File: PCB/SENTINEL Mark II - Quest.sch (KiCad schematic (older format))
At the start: 22 parts, among them J10 External, J7 SERVO1, J8 SERVO2, J9 SENSOR, U3 STM32F103CBTx, Y1 8MHz/20pF

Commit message: Footprint Assigned
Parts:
- C11, C12, C13, C14, C15, C16, C17: footprint (none) -> Capacitor_SMD:C_0805_2012Metric
- D4: footprint (none) -> LED_SMD:LED_0805_2012Metric
- FB2, FB3, FB4: footprint (none) -> Inductor_SMD:L_0805_2012Metric
- J10: footprint (none) -> Connector_PinHeader_2.54mm:PinHeader_1x04_P2.54mm_Vertical
- J7, J8, JP1: footprint (none) -> Connector_PinHeader_2.54mm:PinHeader_1x03_P2.54mm_Vertical
- J9: footprint (none) -> Connector_PinHeader_2.54mm:PinHeader_1x09_P2.54mm_Horizontal
- R12, R7, R8, R9: footprint (none) -> Resistor_SMD:R_0805_2012Metric
- Y1: footprint (none) -> Crystal:Crystal_SMD_3225-4Pin_3.2x2.5mm_HandSoldering; symbol Device:Crystal -> Device:Crystal_GND24
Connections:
- net GND: now also C11.1, C12.1, Y1.2, Y1.4; no longer C11.2, C12.2
- net at U3.5 (PD0), Y1.1: now also C12.2; no longer C11.1
- new net: C11.2, U3.6 (PD1), Y1.3
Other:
- moved on the sheet: C11, C12
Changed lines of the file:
@@
 F 0 "C15" H 7040 2296 50  0000 L CNN
 F 1 "1uF" H 7040 2205 50  0000 L CNN
-F 2 "" H 6963 2100 50  0001 C CNN
+F 2 "Capacitor_SMD:C_0805_2012Metric" H 6963 2100 50  0001 C CNN
 F 3 "~" H 6925 2250 50  0001 C CNN
 	1    6925 2250
@@
 F 0 "C16" H 7565 2296 50  0000 L CNN
 F 1 "1uF" H 7565 2205 50  0000 L CNN
-F 2 "" H 7488 2100 50  0001 C CNN
+F 2 "Capacitor_SMD:C_0805_2012Metric" H 7488 2100 50  0001 C CNN
 F 3 "~" H 7450 2250 50  0001 C CNN
 	1    7450 2250
@@
 F 0 "C17" H 8065 2296 50  0000 L CNN
 F 1 "1uF" H 8065 2205 50  0000 L CNN
-F 2 "" H 7988 2100 50  0001 C CNN
+F 2 "Capacitor_SMD:C_0805_2012Metric" H 7988 2100 50  0001 C CNN
 F 3 "~" H 7950 2250 50  0001 C CNN
 	1    7950 2250
@@
 F 0 "C14" H 6515 2296 50  0000 L CNN
 F 1 "1uF" H 6515 2205 50  0000 L CNN
-F 2 "" H 6438 2100 50  0001 C CNN
+F 2 "Capacitor_SMD:C_0805_2012Metric" H 6438 2100 50  0001 C CNN
 F 3 "~" H 6400 2250 50  0001 C CNN
 	1    6400 2250
@@
 F 0 "R8" H 5050 1675 50  0000 L CNN
 F 1 "10K" V 5000 1575 50  0000 L CNN
-F 2 "" V 4930 1650 50  0001 C CNN
+F 2 "Resistor_SMD:R_0805_2012Metric" V 4930 1650 50  0001 C CNN
 F 3 "~" H 5000 1650 50  0001 C CNN
 	1    5000 1650
@@
 Wire Wire Line
 	5000 3700 5000 3600
-Wire Wire Line
-	4375 3700 5000 3700
-Wire Wire Line
-	4375 3400 5000 3400
-$Comp
-L Device:Crystal Y1
+$Comp
+L Device:Crystal_GND24 Y1
 U 1 1 5F6E91F4
-P 4375 3550
+P 4425 3550
 AR Path="/5F6E91F4" Ref="Y1"  Part="1"
 AR Path="/5F584CC7/5F6E91F4" Ref="Y?"  Part="1"
-F 0 "Y1" V 4329 3681 50  0000 L CNN
-F 1 "8MHz/20pF" V 4420 3681 50  0000 L CNN
-F 2 "" H 4375 3550 50  0001 C CNN
-F 3 "~" H 4375 3550 50  0001 C CNN
-	1    4375 3550
+F 0 "Y1" V 4450 2800 50  0000 L CNN
+F 1 "8MHz/20pF" V 4525 2800 50  0000 L CNN
+F 2 "Crystal:Crystal_SMD_3225-4Pin_3.2x2.5mm_HandSoldering" H 4425 3550 50  0001 C CNN
+F 3 "~" H 4425 3550 50  0001 C CNN
+	1    4425 3550
 	0    1    1    0
 $EndComp
@@
 L Device:C C11
 U 1 1 5F6E91FA
-P 4125 3400
+P 4275 3850
 AR Path="/5F6E91FA" Ref="C11"  Part="1"
 AR Path="/5F584CC7/5F6E91FA" Ref="C?"  Part="1"
-F 0 "C11" V 3925 3400 50  0000 C CNN
-F 1 "33pF" V 4000 3400 50  0000 C CNN
-F 2 "" H 4163 3250 50  0001 C CNN
-F 3 "~" H 4125 3400 50  0001 C CNN
-	1    4125 3400
-	0    1    1    0
+F 0 "C11" V 4075 3850 50  0000 C CNN
+F 1 "33pF" V 4150 3850 50  0000 C CNN
+F 2 "Capacitor_SMD:C_0805_2012Metric" H 4313 3700 50  0001 C CNN
+F 3 "~" H 4275 3850 50  0001 C CNN
+	1    4275 3850
+	0    -1   -1   0
 $EndComp
 $Comp
 L Device:C C12
 U 1 1 5F6E9200
-P 4125 3700
+P 4275 3225
 AR Path="/5F6E9200" Ref="C12"  Part="1"
 AR Path="/5F584CC7/5F6E9200" Ref="C?"  Part="1"
-F 0 "C12" V 4275 3700 50  0000 C CNN
-F 1 "33pF" V 4350 3700 50  0000 C CNN
-F 2 "" H 4163 3550 50  0001 C CNN
-F 3 "~" H 4125 3700 50  0001 C CNN
-	1    4125 3700
-	0    1    1    0
+F 0 "C12" V 4425 3225 50  0000 C CNN
+F 1 "33pF" V 4500 3225 50  0000 C CNN
+F 2 "Capacitor_SMD:C_0805_2012Metric" H 4313 3075 50  0001 C CNN
+F 3 "~" H 4275 3225 50  0001 C CNN
+	1    4275 3225
+	0    -1   -1   0
 $EndComp
 $Comp
@@
 F 0 "C13" H 5915 2071 50  0000 L CNN
 F 1 "100nF" H 5915 1980 50  0000 L CNN
-F 2 "" H 5838 1875 50  0001 C CNN
+F 2 "Capacitor_SMD:C_0805_2012Metric" H 5838 1875 50  0001 C CNN
 F 3 "~" H 5800 2025 50  0001 C CNN
 	1    5800 2025
@@
 F 0 "R9" H 5850 1775 50  0000 L CNN
 F 1 "10K" V 5800 1650 50  0000 L CNN
-F 2 "" V 5730 1725 50  0001 C CNN
+F 2 "Resistor_SMD:R_0805_2012Metric" V 5730 1725 50  0001 C CNN
 F 3 "~" H 5800 1725 50  0001 C CNN
 	1    5800 1725
@@
 L power:GND #PWR020
 U 1 1 5F6E9221
-P 3975 3550
+P 4125 3550
 AR Path="/5F6E9221" Ref="#PWR020"  Part="1"
 AR Path="/5F584CC7/5F6E9221" Ref="#PWR?"  Part="1"
-F 0 "#PWR020" H 3975 3300 50  0001 C CNN
-F 1 "GND" H 3980 3377 50  0000 C CNN
-F 2 "" H 3975 3550 50  0001 C CNN
-F 3 "" H 3975 3550 50  0001 C CNN
-	1    3975 3550
+F 0 "#PWR020" H 4125 3300 50  0001 C CNN
+F 1 "GND" V 4125 3375 50  0000 C CNN
+F 2 "" H 4125 3550 50  0001 C CNN
+F 3 "" H 4125 3550 50  0001 C CNN
+	1    4125 3550
 	0    1    1    0
 $EndComp
-Wire Wire Line
-	3975 3400 3975 3550
-Connection ~ 3975 3550
-Wire Wire Line
-	3975 3550 3975 3700
-Wire Wire Line
-	4275 3400 4375 3400
-Connection ~ 4375 3400
-Wire Wire Line
-	4275 3700 4375 3700
-Connection ~ 4375 3700
 Text Label 5000 5100 2    50   ~ 0
 DISC
@@
 F 0 "R7" H 4700 1675 50  0000 L CNN
 F 1 "330" V 4900 1575 50  0000 L CNN
-F 2 "" V 4830 1650 50  0001 C CNN
+F 2 "Resistor_SMD:R_0805_2012Metric" V 4830 1650 50  0001 C CNN
 F 3 "~" H 4900 1650 50  0001 C CNN
 	1    4900 1650
@@
 F 0 "D4" H 4893 2166 50  0000 C CNN
 F 1 "LED" H 4893 2075 50  0000 C CNN
-F 2 "" H 4900 1950 50  0001 C CNN
+F 2 "LED_SMD:LED_0805_2012Metric" H 4900 1950 50  0001 C CNN
 F 3 "~" H 4900 1950 50  0001 C CNN
 	1    4900 1950
@@
 F 0 "J9" H 7505 3792 50  0000 L CNN
 F 1 "SENSOR" H 7505 3701 50  0000 L CNN
-F 2 "" H 7425 3750 50  0001 C CNN
+F 2 "Connector_PinHeader_2.54mm:PinHeader_1x09_P2.54mm_Horizontal" H 7425 3750 50  0001 C CNN
 F 3 "~" H 7425 3750 50  0001 C CNN
 	1    7425 3750
@@
 Wire Wire Line
 	7700 2400 7950 2400
-Text Notes 1925 3675 0    50   ~ 0
+Text Notes 1250 3650 0    50   ~ 0
 Typ. Cstray = 3pF\nCa(pF) = Cb(pF) = 2*CL(pF) - 2*Cstray(pF)\nCa = Cb = 2*20 - 2*3 = 34pF
 Wire Notes Line
-	1900 3425 3650 3425
-Wire Notes Line
-	3650 3425 3650 3700
-Wire Notes Line
-	3650 3700 1900 3700
-Wire Notes Line
-	1900 3700 1900 3425
+	1225 3400 2975 3400
+Wire Notes Line
+	2975 3400 2975 3675
+Wire Notes Line
+	2975 3675 1225 3675
+Wire Notes Line
+	1225 3675 1225 3400
 Text Label 7225 3450 2    50   ~ 0
 PWM_LED
@@
 F 0 "J8" H 2593 2892 50  0000 C CNN
 F 1 "SERVO2" H 2593 2801 50  0000 C CNN
-F 2 "" H 2675 2575 50  0001 C CNN
+F 2 "Connector_PinHeader_2.54mm:PinHeader_1x03_P2.54mm_Vertical" H 2675 2575 50  0001 C CNN
 F 3 "~" H 2675 2575 50  0001 C CNN
 	1    2675 2575
@@
 F 0 "J7" H 2593 1700 50  0000 C CNN
 F 1 "SERVO1" H 2593 1791 50  0000 C CNN
-F 2 "" H 2675 2025 50  0001 C CNN
+F 2 "Connector_PinHeader_2.54mm:PinHeader_1x03_P2.54mm_Vertical" H 2675 2025 50  0001 C CNN
 F 3 "~" H 2675 2025 50  0001 C CNN
 	1    2675 2025
@@
 F 0 "FB4" V 6975 1575 50  0000 C CNN
 F 1 "1A" V 7050 1575 50  0000 C CNN
-F 2 "" V 7055 1675 50  0001 C CNN
+F 2 "Inductor_SMD:L_0805_2012Metric" V 7055 1675 50  0001 C CNN
 F 3 "~" H 7125 1675 50  0001 C CNN
 	1    7125 1675
@@
 F 0 "FB3" V 6950 1550 50  0000 C CNN
 F 1 "1A" V 7025 1550 50  0000 C CNN
-F 2 "" V 7055 1400 50  0001 C CNN
+F 2 "Inductor_SMD:L_0805_2012Metric" V 7055 1400 50  0001 C CNN
 F 3 "~" H 7125 1400 50  0001 C CNN
 	1    7125 1400
@@
 F 0 "FB2" V 2825 1700 50  0000 C CNN
 F 1 "1A" V 2900 1700 50  0000 C CNN
-F 2 "" V 2930 1550 50  0001 C CNN
+F 2 "Inductor_SMD:L_0805_2012Metric" V 2930 1550 50  0001 C CNN
 F 3 "~" H 3000 1550 50  0001 C CNN
 	1    3000 1550
@@
 F 0 "R12" V 3900 1925 50  0000 C CNN
 F 1 "10K" V 3975 1925 50  0000 C CNN
-F 2 "" V 3905 1925 50  0001 C CNN
+F 2 "Resistor_SMD:R_0805_2012Metric" V 3905 1925 50  0001 C CNN
 F 3 "~" H 3975 1925 50  0001 C CNN
 	1    3975 1925
@@
 F 0 "JP1" V 4321 1991 50  0000 L CNN
 F 1 "BOOT0" V 4230 1991 50  0000 L CNN
-F 2 "" H 4275 1925 50  0001 C CNN
+F 2 "Connector_PinHeader_2.54mm:PinHeader_1x03_P2.54mm_Vertical" H 4275 1925 50  0001 C CNN
 F 3 "~" H 4275 1925 50  0001 C CNN
 	1    4275 1925
@@
 F 0 "J10" H 7505 4892 50  0000 L CNN
 F 1 "External" H 7505 4801 50  0000 L CNN
-F 2 "" H 7425 4900 50  0001 C CNN
+F 2 "Connector_PinHeader_2.54mm:PinHeader_1x04_P2.54mm_Vertical" H 7425 4900 50  0001 C CNN
 F 3 "~" H 7425 4900 50  0001 C CNN
 	1    7425 4900
@@
 Text Label 7225 5000 2    50   ~ 0
 5V
+$Comp
+L power:GND #PWR0112
+U 1 1 5F69E38C
+P 4625 3550
+AR Path="/5F69E38C" Ref="#PWR0112"  Part="1"
+AR Path="/5F584CC7/5F69E38C" Ref="#PWR?"  Part="1"
+F 0 "#PWR0112" H 4625 3300 50  0001 C CNN
+F 1 "GND" V 4625 3350 50  0000 C CNN
+F 2 "" H 4625 3550 50  0001 C CNN
+F 3 "" H 4625 3550 50  0001 C CNN
+	1    4625 3550
+	0    -1   -1   0
+$EndComp
+Wire Wire Line
+	3000 3900 3000 4200
+Wire Wire Line
+	4425 3400 5000 3400
+Wire Wire Line
+	5000 3700 4425 3700
+Wire Wire Line
+	4425 3850 4425 3700
+Connection ~ 4425 3700
+Wire Wire Line
+	4425 3225 4425 3400
+Connection ~ 4425 3400
+Wire Wire Line
+	4125 3225 4125 3550
+Wire Wire Line
+	4125 3550 4125 3850
+Connection ~ 4125 3550
+Wire Wire Line
+	4225 3550 4125 3550
 $EndSCHEMATC

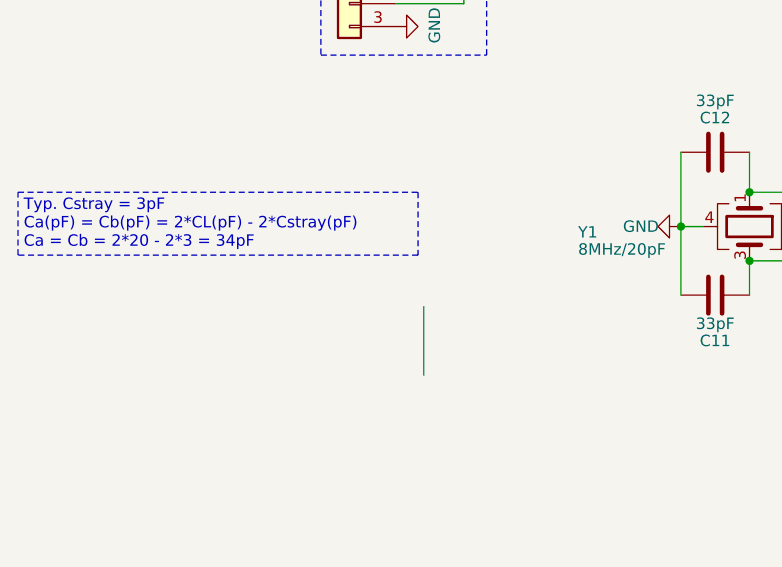
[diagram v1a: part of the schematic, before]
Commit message: KICAD
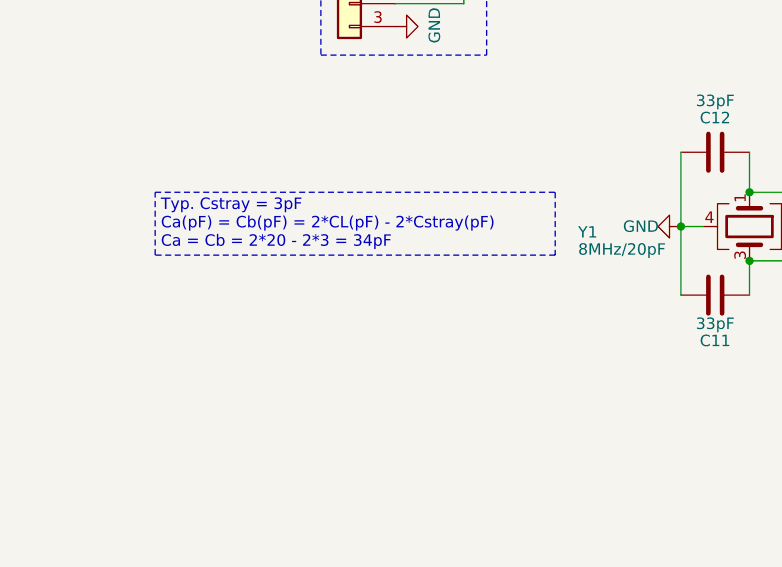
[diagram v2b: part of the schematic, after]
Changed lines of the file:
@@
 Wire Wire Line
 	7700 2400 7950 2400
-Text Notes 1250 3650 0    50   ~ 0
+Text Notes 1850 3650 0    50   ~ 0
 Typ. Cstray = 3pF\nCa(pF) = Cb(pF) = 2*CL(pF) - 2*Cstray(pF)\nCa = Cb = 2*20 - 2*3 = 34pF
 Wire Notes Line
-	1225 3400 2975 3400
-Wire Notes Line
-	2975 3400 2975 3675
-Wire Notes Line
-	2975 3675 1225 3675
-Wire Notes Line
-	1225 3675 1225 3400
+	1825 3400 3575 3400
+Wire Notes Line
+	3575 3400 3575 3675
+Wire Notes Line
+	3575 3675 1825 3675
+Wire Notes Line
+	1825 3675 1825 3400
 Text Label 7225 3450 2    50   ~ 0
 PWM_LED
@@
 $EndComp
 Wire Wire Line
-	3000 3900 3000 4200
-Wire Wire Line
 	4425 3400 5000 3400
